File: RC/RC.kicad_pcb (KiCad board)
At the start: 2 copper layers, 120 x 95 mm, 45 parts, among them J1 BEC, J10 CJVL53L0XV2, J11 CJMCU-20948, J12 A3144 REMOTE, J2 ESP32L, J3 ESP32R, J4 BuckIn-, J5 BuckIn+, J6 BuckOut-, J7 BuckOut+, J8 VBAT_SENSE_IN, J9 3V3 LINK, M1 MG90

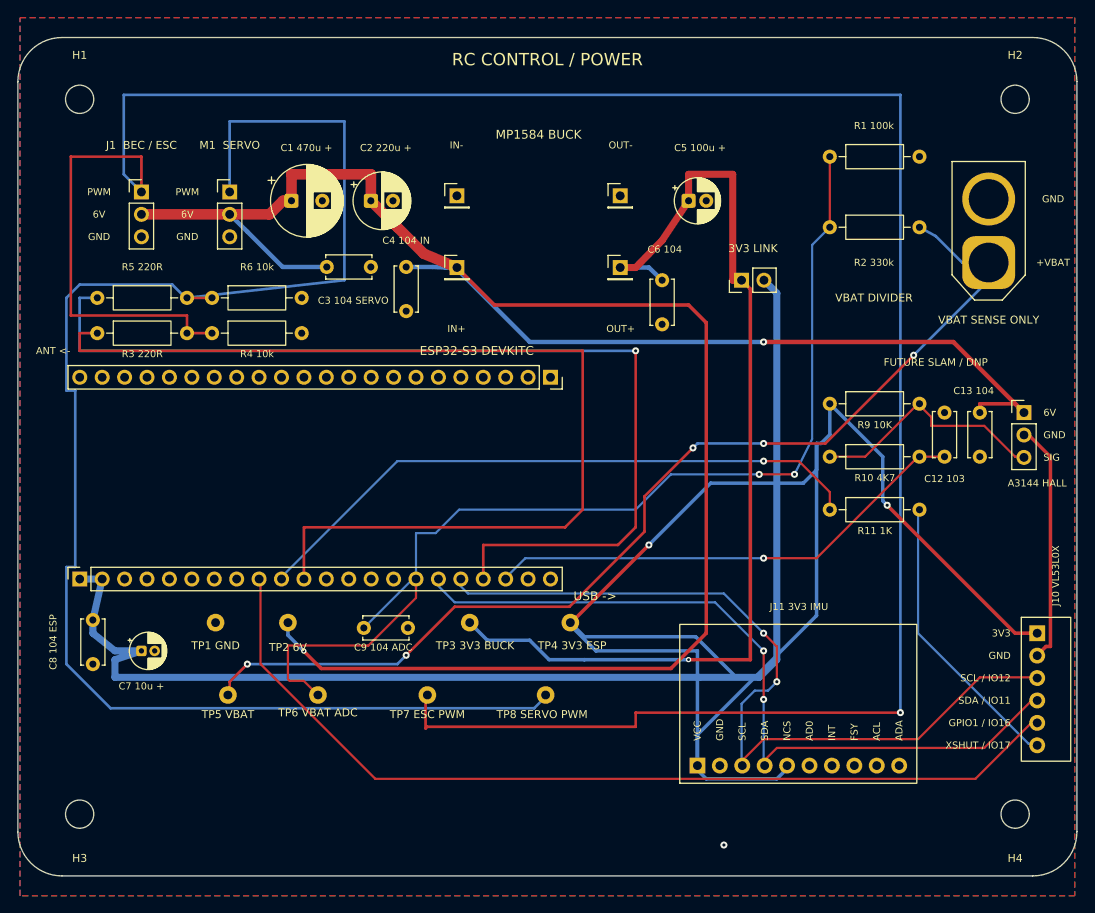
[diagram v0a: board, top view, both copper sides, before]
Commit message: Release RC carrier PCB v1.0 for fabrication
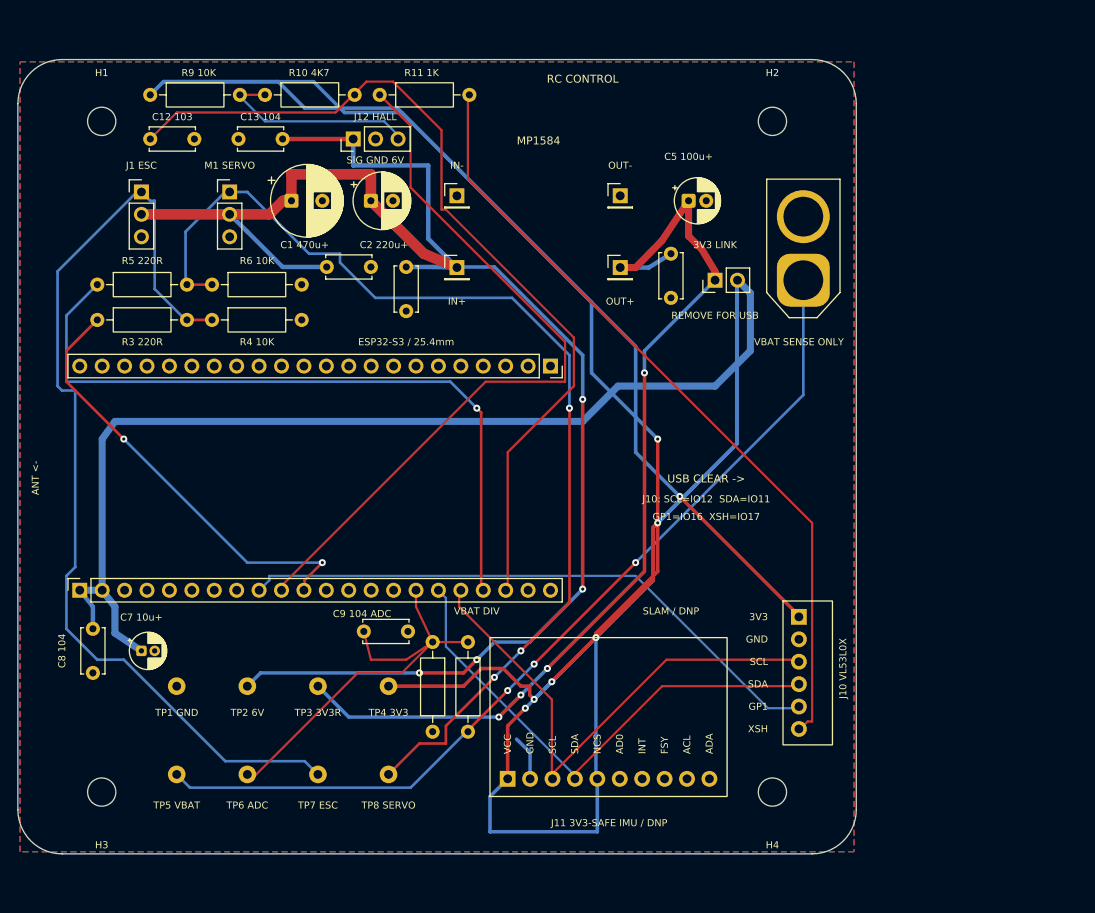
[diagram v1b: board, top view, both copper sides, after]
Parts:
- moved C12 96.9 mm to (35.0, 94.0), turned to 0 degrees
- moved C13 84.9 mm to (50.0, 94.0), turned to 180 degrees
- moved R9 84.6 mm to (35.0, 89.0)
- moved J12 82.1 mm to (58.0, 94.0), turned to 90 degrees
- moved R10 76.0 mm to (48.0, 89.0)
- moved R1 71.1 mm to (67.0, 151.0), turned to -90 degrees
- moved R11 69.4 mm to (61.0, 89.0)
- moved R2 62.4 mm to (71.0, 151.0), turned to -90 degrees
- moved H2 27.6 mm to (105.5, 92.0)
- moved H4 27.6 mm to (105.5, 168.0)
- moved J10 27.1 mm to (108.5, 148.2)
- moved TP4 21.8 mm to (62.0, 156.0)
- moved J11 21.6 mm to (75.5, 166.5)
- moved J8 21.1 mm to (109.0, 110.0)
- moved TP8 19.9 mm to (62.0, 166.0)
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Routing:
- net +3.3V: track 327.7 -> 516.1 mm, vias 2 -> 7
- net /PWM_ESC_OUT: track 277.2 -> 111.0 mm, vias 1 -> 0
- net +6V: track 260.5 -> 184.8 mm, vias 2 -> 4
- net /VBAT_SENSE: track 123.2 -> 48.4 mm, vias 2 -> 0
- net /PWM_ESC: track 117.3 -> 49.9 mm, vias 0 -> 2
- net /VL_XSHUT: track 33.0 -> 89.4 mm
- net /PWM_SERVO_OUT: track 175.6 -> 120.4 mm, vias 0 -> 3
- net /IO14: track 55.9 -> 100.2 mm, vias 1 -> 0
- net /IO16: track 106.0 -> 68.5 mm
- net /IO12: track 93.8 -> 60.4 mm, vias 2 -> 0
- net /PWM_SERVO: track 113.0 -> 81.2 mm
- net /IO11: track 88.6 -> 58.7 mm, vias 2 -> 0
- net GND: track 27.5 -> 5.15 mm, vias 1 -> 0
- net /VBAT: track 120.2 -> 103.4 mm, vias 5 -> 3
- net /IO17: track 71.5 -> 83.4 mm, vias 1 -> 0
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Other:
- board size 120 x 95 mm -> 95 x 90 mm
- board text added: "3V3"
- board text added: "C1 470u+"
- board text added: "C2 220u+"
- board text added: "C5 100u+"
- board text added: "C7 10u+"
- board text added: "C8 104"
- board text added: "ESP32-S3 / 25.4mm"
- board text added: "GP1"
- board text added: "GP1=IO16 XSH=IO17"
- board text added: "J1 ESC"
- board text added: "J10 VL53L0X"
- board text added: "J10: SCL=IO12 SDA=IO11"
- board text added: "J11 3V3-SAFE IMU / DNP"
- board text added: "J12 HALL"
- board text added: "MP1584"
- board text added: "R4 10K"
- board text added: "R6 10K"
- board text added: "RC CONTROL"
- board text added: "REMOVE FOR USB"
- board text added: "SCL"
- board text added: "SDA"
- board text added: "SIG GND 6V"
- board text added: "SLAM / DNP"
- board text added: "TP3 3V3R"
- board text added: "TP4 3V3"
- board text added: "TP6 ADC"
- board text added: "TP7 ESC"
- board text added: "TP8 SERVO"
- board text added: "USB CLEAR ->"
- board text added: "VBAT DIV"
- board text added: "XSH"
- board text removed: "+VBAT"
- board text removed: "6V"
- board text removed: "A3144 HALL"
- board text removed: "C1 470u +"
- board text removed: "C2 220u +"
- board text removed: "C3 104 SERVO"
- board text removed: "C4 104 IN"
- board text removed: "C5 100u +"
- board text removed: "C6 104"
- board text removed: "C7 10u +"
- board text removed: "C8 104 ESP"
- board text removed: "ESP32-S3 DEVKITC"
- board text removed: "FUTURE SLAM / DNP"
- board text removed: "J1 BEC / ESC"
- board text removed: "J11 3V3 IMU"
- board text removed: "MP1584 BUCK"
- board text removed: "PWM"
- board text removed: "R1 100k"
- board text removed: "R2 330k"
- board text removed: "R4 10k"
- board text removed: "R6 10k"
- board text removed: "RC CONTROL / POWER"
- board text removed: "SIG"
- board text removed: "TP3 3V3 BUCK"
- board text removed: "TP4 3V3 ESP"
- board text removed: "TP6 VBAT ADC"
- board text removed: "TP7 ESC PWM"
- board text removed: "TP8 SERVO PWM"
- board text removed: "USB ->"
- board text removed: "VBAT DIVIDER"
